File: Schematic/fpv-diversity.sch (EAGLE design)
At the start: 32 parts, among them U1 LM1881M/NOPB, U2 LM1881M/NOPB, U3 LM1881M/NOPB, U4 MAX4545CAP+

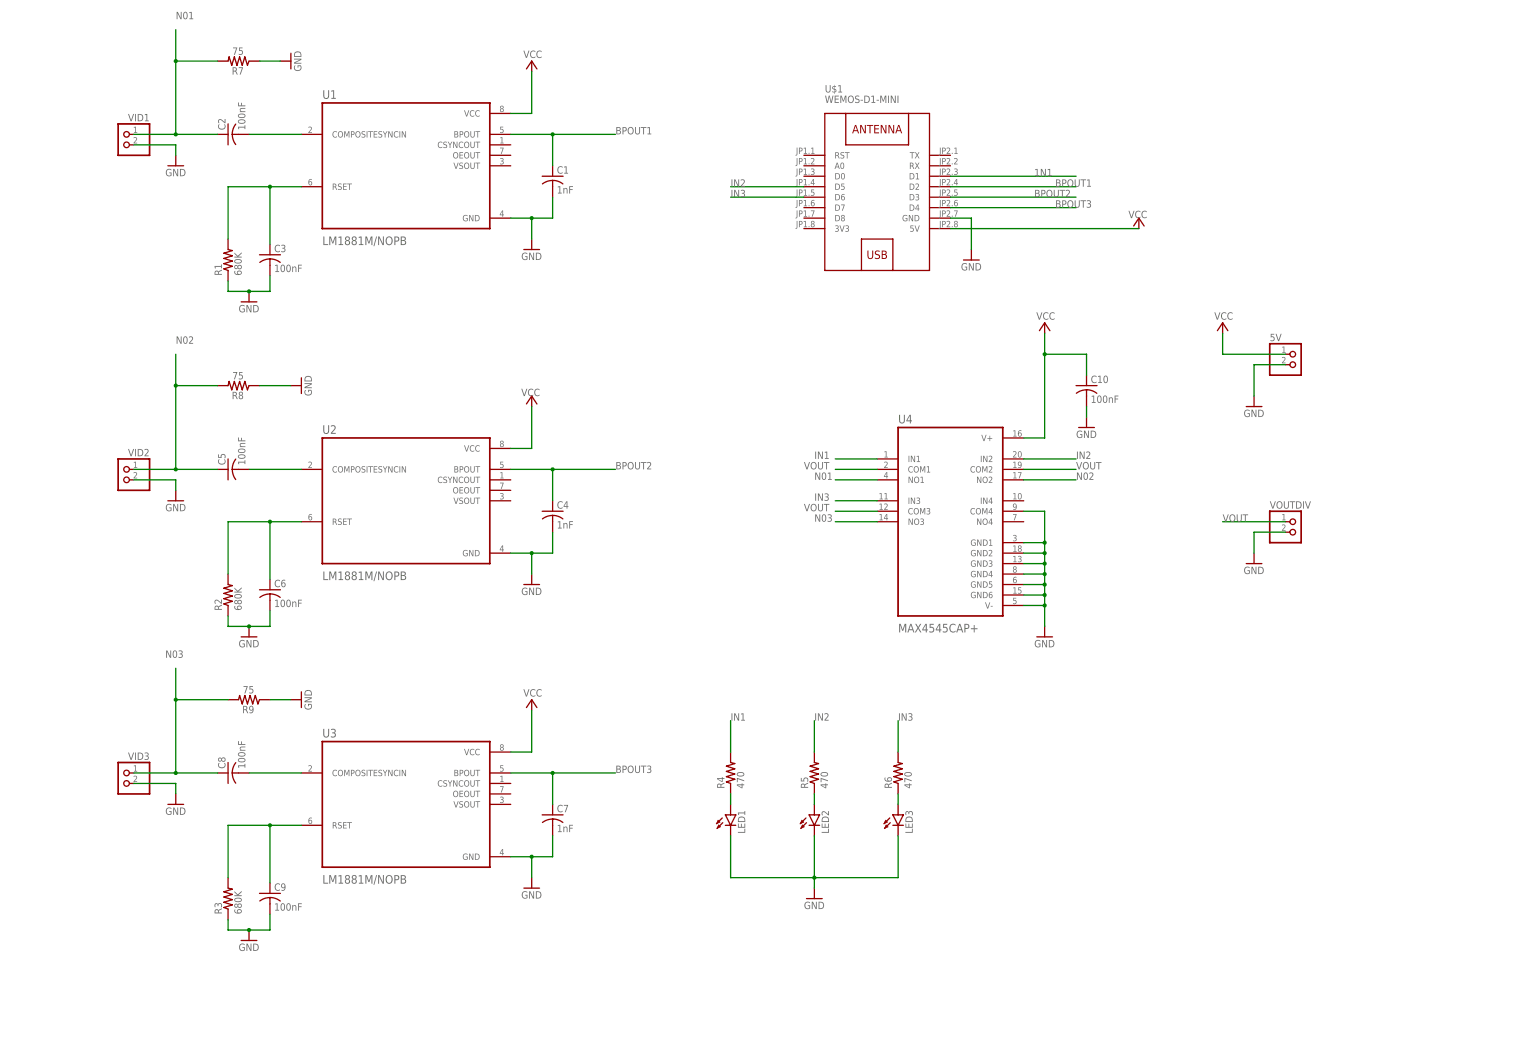
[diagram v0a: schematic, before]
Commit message: PCB updates
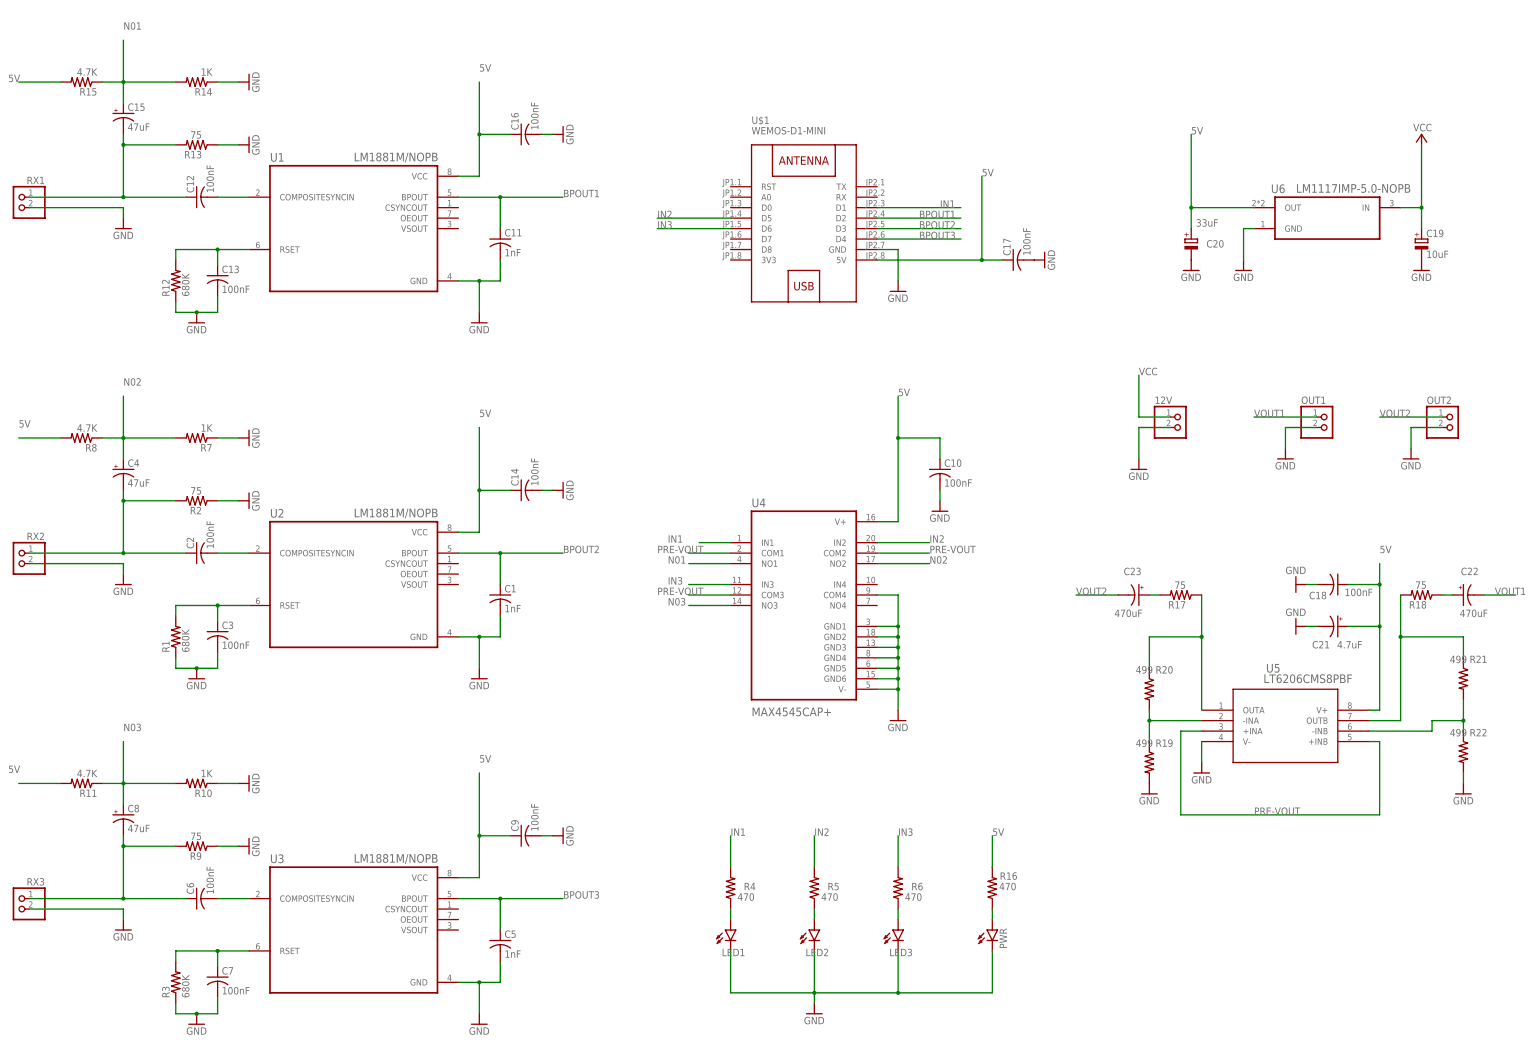
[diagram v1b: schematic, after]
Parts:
- removed 5V, VID1, VID2, VID3, VOUTDIV: (no value), pinhead:PINHD-1X2
- added 12V, OUT1, OUT2, RX1, RX2, RX3: (no value), pinhead:PINHD-1X2
- added C11: 1nF, rcl:C-USC0805
- added C12, C13, C14, C16, C17, C18: 100nF, rcl:C-USC0805
- added C15: 47uF, rcl:CPOL-USCT3528
- added C19: 10uF, rcl:CPOL-EUD
- added C20: 33uF, rcl:CPOL-EUD
- added C21: 4.7uF, rcl:CPOL-USCT3528
- added C22, C23: 470uF, rcl:CPOL-USCT3528
- added PWR: (no value), led:LEDCHIP-LED0805
- added R10, R14: 1K, rcl:R-US_R1206
- added R11, R15: 4.7K, rcl:R-US_R1206
- added R12: 680K, rcl:R-US_R1206
- added R13, R17, R18: 75, rcl:R-US_R1206
- added R16: 470, rcl:R-US_R1206
- added R19, R20, R21, R22: 499, rcl:R-US_R1206
- added U5: LT6206CMS8PBF, LT6206CMS8PBF:LT6206CMS8PBF
- added U6: LM1117IMP-5.0-NOPB, LM1117IMP-5.0-NOPB:LM1117IMP-5.0-NOPB
- C1, C10, C2, C3, C6, C9: device rcl:C-USC0402 -> rcl:C-USC0805
- C4: value 1nF -> 47uF; device rcl:C-USC0402 -> rcl:CPOL-USCT3528
- C5: value 100nF -> 1nF; device rcl:C-USC0402 -> rcl:C-USC0805
- C7: value 1nF -> 100nF; device rcl:C-USC0402 -> rcl:C-USC0805
- C8: value 100nF -> 47uF; device rcl:C-USC0402 -> rcl:CPOL-USCT3528
- R1, R3, R4, R5, R6, R9: device rcl:R-US_R0603 -> rcl:R-US_R1206
- R2: value 680K -> 75; device rcl:R-US_R0603 -> rcl:R-US_R1206
- R7: value 75 -> 1K; device rcl:R-US_R0603 -> rcl:R-US_R1206
- R8: value 75 -> 4.7K; device rcl:R-US_R0603 -> rcl:R-US_R1206
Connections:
- removed net 1N1: U$1.D1
- removed net N$6: C8.2, U3.COMPOSITESYNCIN
- removed net VOUT: U4.COM1, U4.COM2, U4.COM3, VOUTDIV.1
- new net 5V: C10.1, C14.1, C16.1, C17.1, C18.1, C20.+, C21.+, C9.1, R11.2, R15.2, R16.2, R8.2, U$1.5V, U1.VCC, U2.VCC, U3.VCC, U4.V+, U5.V+, U6.OUT
- new net N$10: C13.1, R12.2, U1.RSET
- new net N$11: C12.2, U1.COMPOSITESYNCIN
- new net N$12: R19.1, R20.2, U5.-INA
- new net N$13: R18.2, R21.1, U5.OUTB
- new net N$14: R21.2, R22.1, U5.-INB
- new net N$15: R17.1, R20.1, U5.OUTA
- new net N$16: C22.+, R18.1
- new net N$17: C23.+, R17.2
- new net PRE-VOUT: U4.COM1, U4.COM2, U4.COM3, U5.+INA, U5.+INB
- new net VID1: C12.1, C15.-, R13.2, RX1.1
- new net VID2: C2.1, C4.-, R2.2, RX2.1
- new net VID3: C6.1, C8.-, R9.2, RX3.1
- new net VOUT1: C22.-, OUT1.1
- new net VOUT2: C23.-, OUT2.1
- net BPOUT1: now also C11.1; no longer C1.1
- net BPOUT2: now also C1.1; no longer C4.1
- net BPOUT3: now also C5.1; no longer C7.1
- net GND: now also 12V.2, C11.2, C13.2, C14.2, C16.2, C17.2, C18.2, C19.-, C20.-, C21.-, C5.2, OUT1.2, OUT2.2, PWR.C, R10.1, R12.1, R13.1, R14.1, R19.2, R22.2, RX1.2, RX2.2, RX3.2, U5.V-, U6.GND; no longer 5V.2, C4.2, C6.2, R8.1, VID1.2, VID2.2, VID3.2, VOUTDIV.2
- net IN1: now also U$1.D1
- net N$1: now also C7.1, R3.2, U3.RSET; no longer C2.2, U1.COMPOSITESYNCIN
- net N$2: now also C3.1, R1.2; no longer C6.1, R2.2
- net N$3: now also C2.2, U2.COMPOSITESYNCIN; no longer C3.1, R1.2, U1.RSET
- net N$4: now also PWR.A, R16.1; no longer C5.2, U2.COMPOSITESYNCIN
- net N$5: now also C6.2, U3.COMPOSITESYNCIN; no longer C9.1, R3.2, U3.RSET
- net N01: now also C15.+, R14.2, R15.1; no longer C2.1, R7.2, VID1.1
- net N02: now also C4.+, R7.2, R8.1; no longer C5.1, R8.2, VID2.1
- net N03: now also C8.+, R10.2, R11.1; no longer C8.1, R9.2, VID3.1
- net VCC: now also 12V.1, C19.+, U6.IN; no longer 5V.1, C10.1, U$1.5V, U1.VCC, U2.VCC, U3.VCC, U4.V+
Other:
- moved on the sheet: C1, C10, C2, C3, C5, C6, C7, C9, LED1, LED2, LED3, R1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

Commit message: .brd cleanup
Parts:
- C15, C4, C8: device rcl:CPOL-USCT3528 -> rcl:CPOL-USCT3216
- C22, C23: device rcl:CPOL-USCT3528 -> rcl:CPOL-USCT7343
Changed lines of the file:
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@@
 <part name="GND4" library="supply1" library_urn="urn:adsk.eagle:library:371" deviceset="GND" device=""/>
 <part name="U2" library="LM1881M_NOPB" deviceset="LM1881M/NOPB" device="" package3d_urn="urn:adsk.eagle:package:18494142/1"/>
-<part name="C4" library="rcl" library_urn="urn:adsk.eagle:library:334" deviceset="CPOL-US" device="CT3528" package3d_urn="urn:adsk.eagle:package:23325/2" value="47uF"/>
+<part name="C4" library="rcl" library_urn="urn:adsk.eagle:library:334" deviceset="CPOL-US" device="CT3216" package3d_urn="urn:adsk.eagle:package:23327/2" value="47uF"/>
 <part name="R7" library="rcl" library_urn="urn:adsk.eagle:library:334" deviceset="R-US_" device="R1206" package3d_urn="urn:adsk.eagle:package:23540/2" value="1K"/>
 <part name="GND5" library="supply1" library_urn="urn:adsk.eagle:library:371" deviceset="GND" device=""/>
@@
 <part name="GND9" library="supply1" library_urn="urn:adsk.eagle:library:371" deviceset="GND" device=""/>
 <part name="U3" library="LM1881M_NOPB" deviceset="LM1881M/NOPB" device="" package3d_urn="urn:adsk.eagle:package:18494142/1"/>
-<part name="C8" library="rcl" library_urn="urn:adsk.eagle:library:334" deviceset="CPOL-US" device="CT3528" package3d_urn="urn:adsk.eagle:package:23325/2" value="47uF"/>
+<part name="C8" library="rcl" library_urn="urn:adsk.eagle:library:334" deviceset="CPOL-US" device="CT3216" package3d_urn="urn:adsk.eagle:package:23327/2" value="47uF"/>
 <part name="R10" library="rcl" library_urn="urn:adsk.eagle:library:334" deviceset="R-US_" device="R1206" package3d_urn="urn:adsk.eagle:package:23540/2" value="1K"/>
 <part name="GND12" library="supply1" library_urn="urn:adsk.eagle:library:371" deviceset="GND" device=""/>
@@
 <part name="GND21" library="supply1" library_urn="urn:adsk.eagle:library:371" deviceset="GND" device=""/>
 <part name="U1" library="LM1881M_NOPB" deviceset="LM1881M/NOPB" device="" package3d_urn="urn:adsk.eagle:package:18494142/1"/>
-<part name="C15" library="rcl" library_urn="urn:adsk.eagle:library:334" deviceset="CPOL-US" device="CT3528" package3d_urn="urn:adsk.eagle:package:23325/2" value="47uF"/>
+<part name="C15" library="rcl" library_urn="urn:adsk.eagle:library:334" deviceset="CPOL-US" device="CT3216" package3d_urn="urn:adsk.eagle:package:23327/2" value="47uF"/>
 <part name="R14" library="rcl" library_urn="urn:adsk.eagle:library:334" deviceset="R-US_" device="R1206" package3d_urn="urn:adsk.eagle:package:23540/2" value="1K"/>
 <part name="GND23" library="supply1" library_urn="urn:adsk.eagle:library:371" deviceset="GND" device=""/>
@@
 <part name="C21" library="rcl" library_urn="urn:adsk.eagle:library:334" deviceset="CPOL-US" device="CT3528" package3d_urn="urn:adsk.eagle:package:23325/2" value="4.7uF"/>
 <part name="GND34" library="supply1" library_urn="urn:adsk.eagle:library:371" deviceset="GND" device=""/>
-<part name="C22" library="rcl" library_urn="urn:adsk.eagle:library:334" deviceset="CPOL-US" device="CT3528" package3d_urn="urn:adsk.eagle:package:23325/2" value="470uF"/>
-<part name="C23" library="rcl" library_urn="urn:adsk.eagle:library:334" deviceset="CPOL-US" device="CT3528" package3d_urn="urn:adsk.eagle:package:23325/2" value="470uF"/>
+<part name="C22" library="rcl" library_urn="urn:adsk.eagle:library:334" deviceset="CPOL-US" device="CT7343" package3d_urn="urn:adsk.eagle:package:23304/2" value="470uF"/>
+<part name="C23" library="rcl" library_urn="urn:adsk.eagle:library:334" deviceset="CPOL-US" device="CT7343" package3d_urn="urn:adsk.eagle:package:23304/2" value="470uF"/>
 </parts>
 <sheets>
